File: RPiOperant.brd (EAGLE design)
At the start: 136 x 94 mm, 69 parts, among them IC1 74LS14N, IC2 74LS14N, J2 POWER_JACK

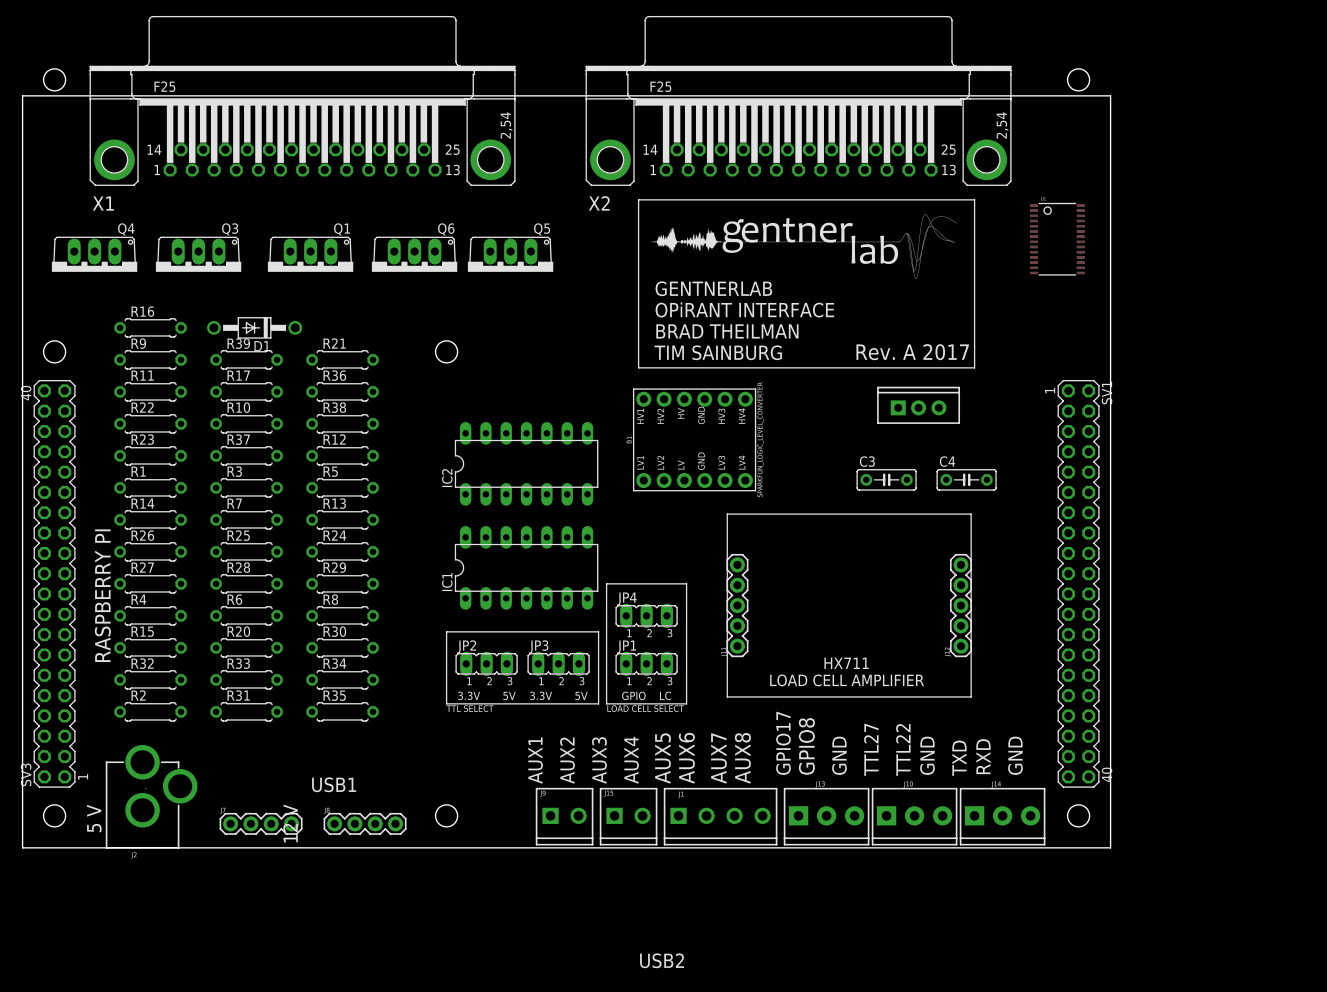
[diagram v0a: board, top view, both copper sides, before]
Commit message: new board layout
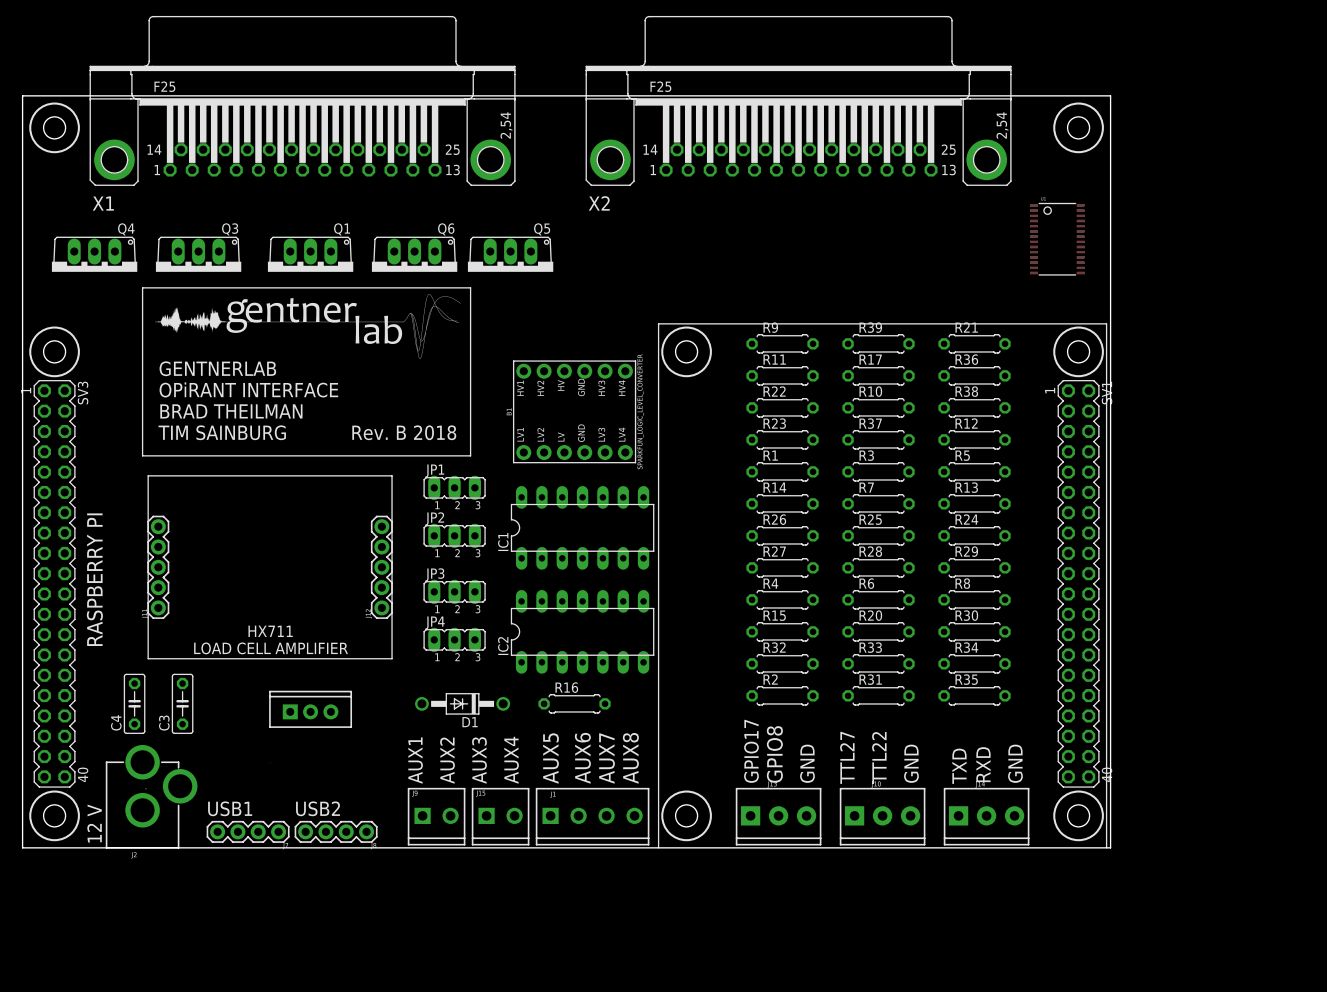
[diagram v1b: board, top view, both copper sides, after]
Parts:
- moved C4 107.7 mm to (14.0, 18.0), turned to 90 degrees
- moved C3 92.3 mm to (20.0, 18.0), turned to 90 degrees
- moved U2 85.0 mm to (36.0, 17.0)
- moved R1 79.0 mm to (95.0, 47.0)
- moved R10 79.0 mm to (107.0, 55.0)
- moved R11 79.0 mm to (95.0, 59.0)
- moved R12 79.0 mm to (119.0, 51.0)
- moved R13 79.0 mm to (119.0, 43.0)
- moved R14 79.0 mm to (95.0, 43.0)
- moved R15 79.0 mm to (95.0, 27.0)
- moved R17 79.0 mm to (107.0, 59.0)
- moved R2 79.0 mm to (95.0, 19.0)
- moved R20 79.0 mm to (107.0, 27.0)
- moved R21 79.0 mm to (119.0, 63.0)
- moved R22 79.0 mm to (95.0, 55.0)
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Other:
- board text added: "Rev. B 2018"
- board text removed: "3.3V 5V"
- board text removed: "5 V"
- board text removed: "GPIO LC"
- board text removed: "LOAD CELL SELECT"
- board text removed: "Rev. A 2017"
- board text removed: "TTL SELECT"

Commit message: revb revisions
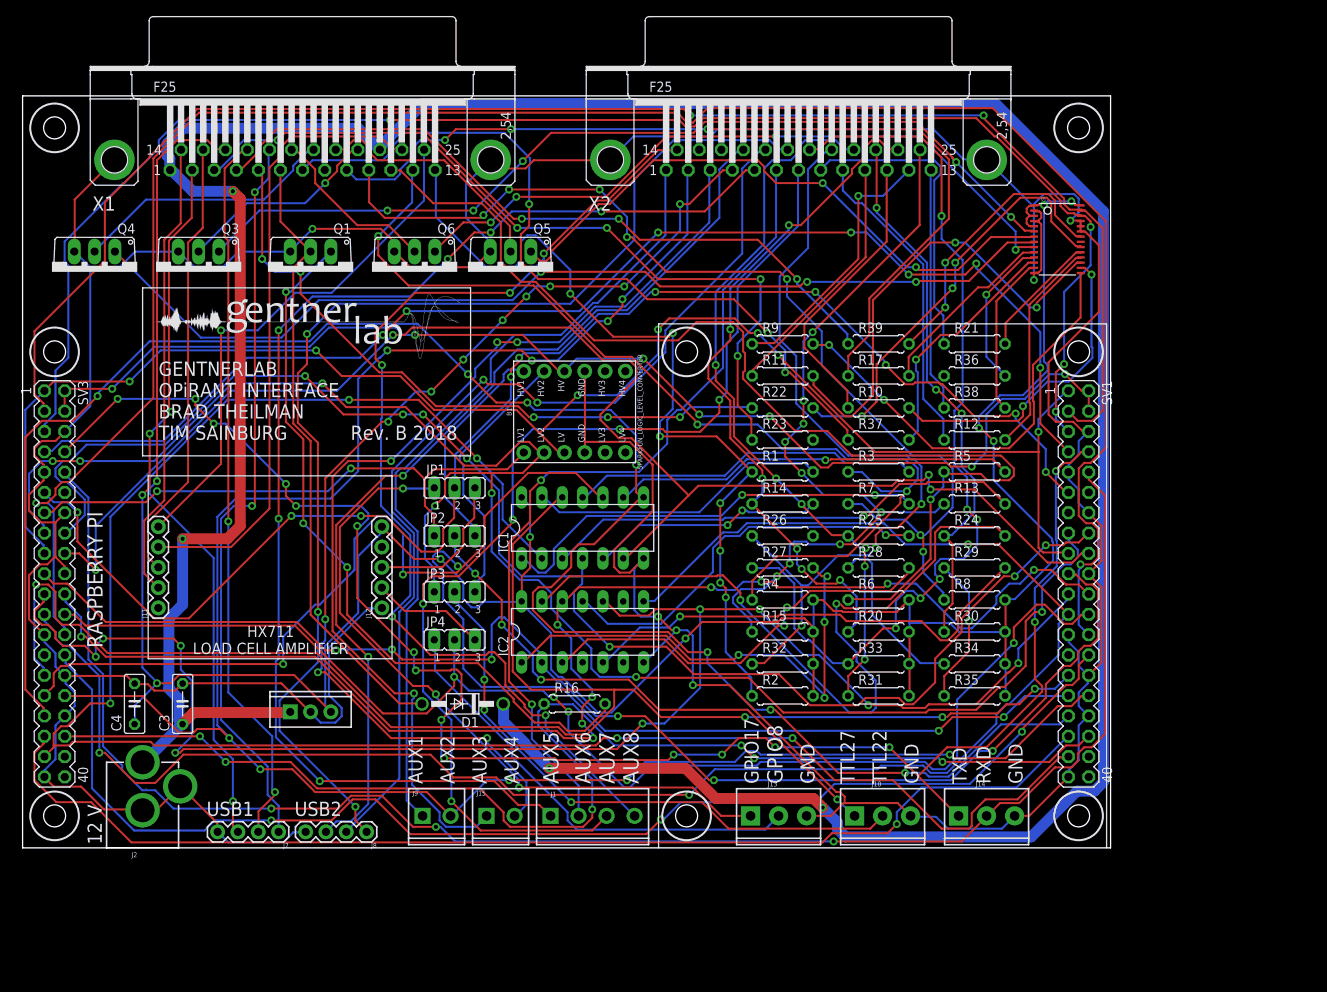
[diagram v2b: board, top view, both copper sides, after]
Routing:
- net GND: track 0.00 -> 590.5 mm, vias 0 -> 6
- net 12V: track 0.00 -> 393.1 mm, vias 0 -> 4
- net +3V3: track 0.00 -> 347.9 mm, vias 0 -> 11
- net AUX2: track 0.00 -> 259.7 mm, vias 0 -> 9
- net GPIO7: track 0.00 -> 255.2 mm, vias 0 -> 2
- net RIGHT_PECK_GPIO: track 0.00 -> 243.1 mm, vias 0 -> 5
- net CENTER_PECK_GPIO: track 0.00 -> 233.9 mm, vias 0 -> 7
- net GPIO22: track 0.00 -> 223.7 mm, vias 0 -> 7
- net IR_5_GPIO: track 0.00 -> 221.8 mm, vias 0 -> 3
- net TXD: track 0.00 -> 213.0 mm, vias 0 -> 16
- net RXD: track 0.00 -> 207.8 mm, vias 0 -> 3
- net LEFT_PECK_GPIO: track 0.00 -> 199.9 mm, vias 0 -> 5
- net RPI_3.3V: track 0.00 -> 197.2 mm, vias 0 -> 7
- net HOPPER_IR_GPIO: track 0.00 -> 196.0 mm, vias 0 -> 4
- net SCL: track 0.00 -> 195.5 mm, vias 0 -> 4
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
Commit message: new board!
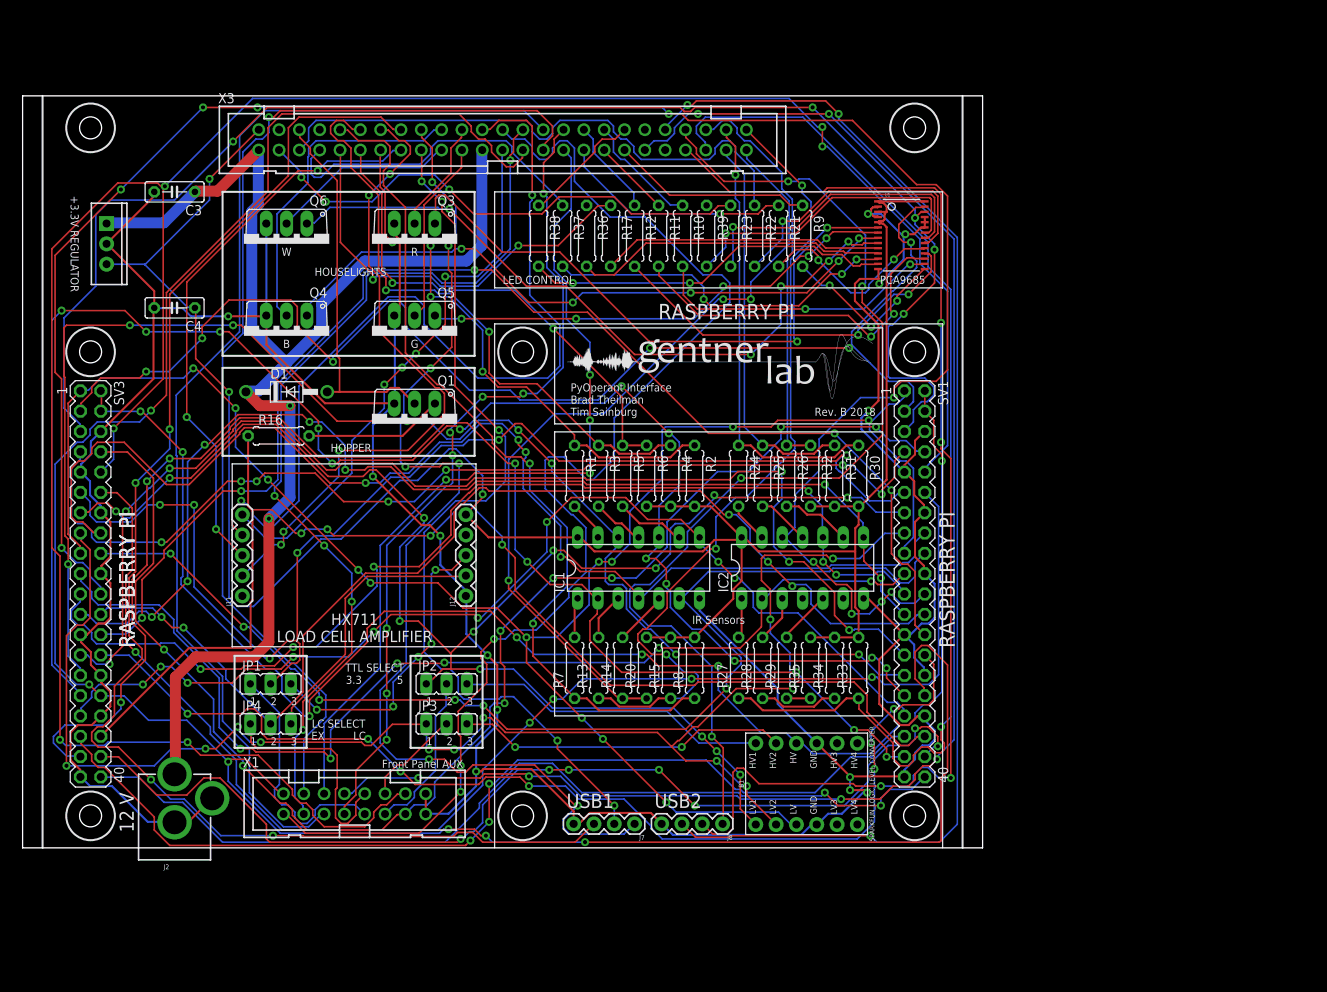
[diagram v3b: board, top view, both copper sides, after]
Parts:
- removed J1: (no value), SparkFun-Connectors:SCREWTERMINAL-3.5MM-4
- removed J10, J13, J14: (no value), SparkFun-Connectors:SCREWTERMINAL-3.5MM-3
- removed J15, J9: (no value), SparkFun-Connectors:SCREWTERMINAL-3.5MM-2
- removed X2: (no value), con-subd:F25HP
- added X3: 2550-, con-3m:PAK100/2500-50
- X1: value (none) -> 2516-; device con-subd:F25HP -> con-3m:PAK100/2500-16
- moved X1 80.8 mm to (41.5, 5.50)
- moved C3 64.0 mm to (19.0, 82.0), turned to 180 degrees
- moved U2 63.8 mm to (10.5, 75.5), turned to 270 degrees
- moved R38 58.6 mm to (64.5, 76.5), turned to 270 degrees
- moved B1 54.8 mm to (98.0, 8.00)
- moved R36 51.6 mm to (70.5, 76.5), turned to 270 degrees
- moved R13 51.3 mm to (72.0, 22.5), turned to 90 degrees
- moved R16 49.9 mm to (32.0, 51.5)
- moved C4 49.8 mm to (19.0, 67.5), turned to 180 degrees
- moved R12 49.6 mm to (76.5, 76.5), turned to 270 degrees
- moved R37 47.0 mm to (67.5, 76.5), turned to 270 degrees
- moved D1 44.8 mm to (33.0, 57.0), turned to 0 degrees
- moved J7 44.5 mm to (76.5, 3.00)
- moved J8 44.5 mm to (87.5, 3.00)
- moved R5 44.0 mm to (75.0, 46.5), turned to 270 degrees
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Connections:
- removed net N$32: J13.1, JP1.1
- removed net N$33: J13.2, JP4.1
- new net GPIO17EXT: JP1.1, X1.9
- new net GPIO8EXT: JP4.1, X1.10
- new net RGB_CUE_B\: X3.4
- net +3V3: now also X3.2; no longer X1.2
- net 12V: now also X3.1, X3.23; no longer X1.1, X1.23
- net AUX1: now also X1.1, X3.26; no longer J9.1, X2.1
- net AUX2: now also X1.2, X3.27; no longer J9.2, X2.2
- net AUX3: now also X1.3, X3.28; no longer J15.1, X2.3
- net AUX4: now also X1.4, X3.29; no longer J15.2, X2.4
- net AUX5: now also X1.5, X3.30; no longer J1.1, X2.5
- net AUX6: now also X1.6, X3.31; no longer J1.2, X2.6
- net AUX7: now also X1.7, X3.32; no longer J1.3, X2.7
- net AUX8: now also X1.8, X3.39; no longer J1.4, X2.14
- net CENTER_IR: now also X3.11; no longer X1.11
- net CENTER_LED: now also X3.8; no longer X1.8
- net GND: now also X1.15, X1.16; no longer J10.3, J13.3, J14.3, X1.G1, X1.G2, X2.G1, X2.G2
- net HOPPER: now also X3.6; no longer X1.6
- net HOPPER_IR: now also X3.13; no longer X1.13
- net HOUSELIGHT_B: now also X3.20; no longer X1.20
- net HOUSELIGHT_G: now also X3.21; no longer X1.21
- net HOUSELIGHT_R: now also X3.22; no longer X1.22
- net HOUSELIGHT_W: now also X3.19; no longer X1.19
- net IR_1: now also X3.50; no longer X2.25
- net IR_2: now also X3.49; no longer X2.24
- net IR_3: now also X3.48; no longer X2.23
- net IR_4: now also X3.47; no longer X2.22
- net IR_5: now also X3.46; no longer X2.21
- net IR_6: now also X3.45; no longer X2.20
- net LED_1: now also X3.38; no longer X2.13
- net LED_2: now also X3.37; no longer X2.12
- net LED_3: now also X3.36; no longer X2.11
- net LED_4: now also X3.35; no longer X2.10
- net LED_5: now also X3.34; no longer X2.9
- net LED_6: now also X3.33; no longer X2.8
- net LEFT_IR: now also X3.12; no longer X1.12
- net LEFT_LED: now also X3.9; no longer X1.9
- net LOADCELL2A+: now also X3.41; no longer X2.16
- net LOADCELL2A-: now also X3.40; no longer X2.15
- net LOADCELLA+: now also X3.15; no longer X1.15
- net LOADCELLA-: now also X3.14; no longer X1.14
- net LOADCELLE+: now also X3.25; no longer X1.25
- net LOADCELLE-: now also X3.24; no longer X1.24
- net RGB_CUE_B: no longer X1.4
- net RGB_CUE_G: now also X3.3; no longer X1.3
- net RGB_CUE_R: now also X3.5; no longer X1.5
- net RIGHT_IR: now also X3.10; no longer X1.10
- net RIGHT_LED: now also X3.7; no longer X1.7
- net RXD: now also X1.14; no longer J14.2
- net TTL22: now also X1.12; no longer J10.2
- net TTL27: now also X1.11; no longer J10.1
- net TXD: now also X1.13; no longer J14.1
- net USB1_D+: now also X3.16; no longer X1.16
- net USB1_D-: now also X3.17; no longer X1.17
- net USB1_VBUS: now also X3.18; no longer X1.18
- net USB2_D+: now also X3.42; no longer X2.17
- net USB2_D-: now also X3.43; no longer X2.18
- net USB2_VBUS: now also X3.44; no longer X2.19
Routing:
- net 12V: track 393.1 -> 165.0 mm, vias 4 -> 2
- net PCM_CLK: track 0.00 -> 168.9 mm, vias 0 -> 5
- net ID_SD: track 0.00 -> 149.3 mm, vias 0 -> 6
- net GPIO27: track 71.8 -> 201.3 mm, vias 2 -> 13
- net PCM_DIN: track 0.00 -> 128.8 mm, vias 0 -> 7
- net PCM_DOUT: track 0.00 -> 115.3 mm, vias 0 -> 2
- net GND: track 590.5 -> 475.2 mm, vias 6 -> 13
- net CENTER_PECK_GPIO: track 233.9 -> 132.7 mm, vias 7 -> 9
- net RXD: track 207.8 -> 308.8 mm, vias 3 -> 6
- net GPIO7: track 255.2 -> 161.4 mm, vias 2 -> 5
- net RGB_CUE_B: track 91.1 -> 0.00 mm, vias 3 -> 0
- net N$3: track 94.3 -> 5.09 mm, vias 2 -> 0
- net N$32: track 87.2 -> 0.00 mm, vias 3 -> 0
- net IR_3_GPIO: track 170.4 -> 251.6 mm, vias 9 -> 10
- net IR_5_GPIO: track 221.8 -> 140.6 mm, vias 3 -> 7
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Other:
- board size 136 x 94 mm -> 120 x 94 mm
- board text added: "+3.3V REGULATOR"
- board text added: "B"
- board text added: "Front Panel AUX"
- board text added: "G"
- board text added: "HOPPER"
- board text added: "HOUSELIGHTS"
- board text added: "IR Sensors"
- board text added: "LC SELECT EX LC"
- board text added: "LED CONTROL"
- board text added: "PCA9685"
- board text added: "PyOperant Interface Brad Theilman Tim Sainburg"
- board text added: "R"
- board text added: "TTL SELECT 3.3 5"
- board text added: "W"
- board text removed: "AUX1"
- board text removed: "AUX2"
- board text removed: "AUX3"
- board text removed: "AUX4"
- board text removed: "AUX5"
- board text removed: "AUX6"
- board text removed: "AUX7"
- board text removed: "AUX8"
- board text removed: "GENTNERLAB OPiRANT INTERFACE BRAD THEILMAN TIM SAINBURG"
- board text removed: "GND"
- board text removed: "GPIO17"
- board text removed: "GPIO8"
- board text removed: "RXD"
- board text removed: "TTL22"
- board text removed: "TTL27"
- board text removed: "TXD"

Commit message: new board
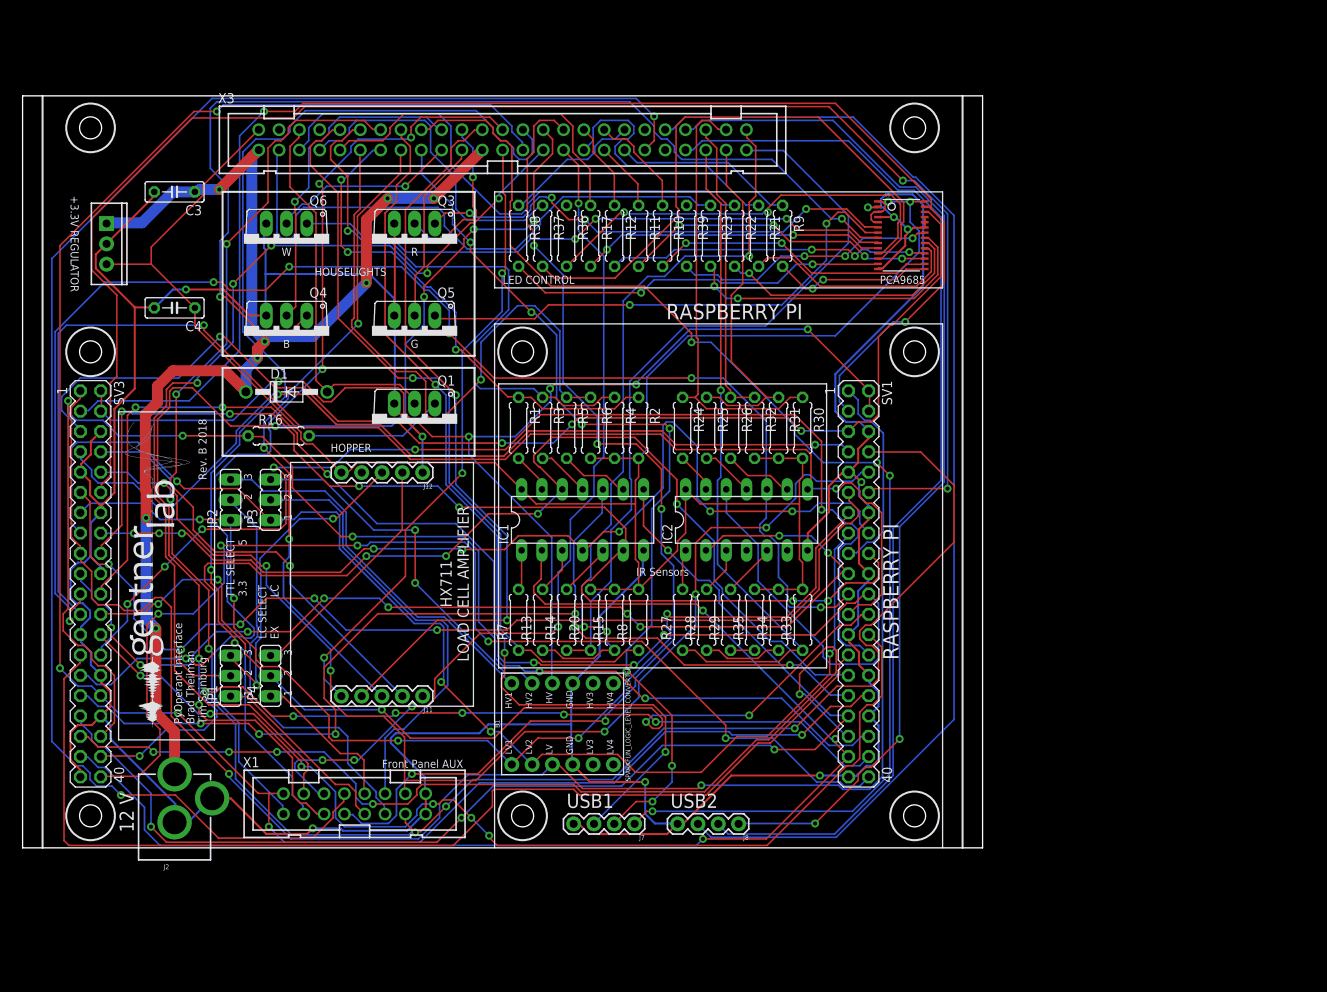
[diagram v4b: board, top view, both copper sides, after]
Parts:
- moved JP3 35.6 mm to (31.0, 43.5), turned to 90 degrees
- moved JP2 35.5 mm to (26.0, 43.5), turned to 90 degrees
- moved B1 31.4 mm to (67.5, 15.5)
- moved J11 25.8 mm to (50.0, 19.0), turned to 180 degrees
- moved J12 16.3 mm to (50.0, 46.9), turned to 180 degrees
- moved IC1 9.22 mm to (70.0, 41.0)
- moved IC2 9.22 mm to (90.5, 41.0)
- moved R1 9.22 mm to (62.0, 52.5)
- moved R13 9.22 mm to (65.0, 28.5)
- moved R14 9.22 mm to (68.0, 28.5)
- moved R15 9.22 mm to (74.0, 28.5)
- moved R2 9.22 mm to (77.0, 52.5)
- moved R20 9.22 mm to (71.0, 28.5)
- moved R24 9.22 mm to (82.5, 52.5)
- moved R25 9.22 mm to (85.5, 52.5)
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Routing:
- net RXD: track 308.8 -> 148.5 mm
- net LEFT_PECK_GPIO: track 203.8 -> 133.7 mm, vias 13 -> 6
- net IR_3_GPIO: track 251.6 -> 183.5 mm, vias 10 -> 6
- net GPIO27: track 201.3 -> 139.4 mm, vias 13 -> 5
- net USB1_D+: track 173.2 -> 116.9 mm, vias 4 -> 3
- net IR_6: track 138.8 -> 84.1 mm
- net HOUSELIGHT_B_GPIO: track 81.8 -> 130.1 mm, vias 5 -> 2
- net TTL22: track 12.5 -> 56.0 mm
- net IR_4_GPIO: track 134.5 -> 177.4 mm
- net AUX2: track 283.5 -> 243.6 mm, vias 6 -> 5
- net RPI_5V: track 193.7 -> 154.6 mm, vias 7 -> 5
- net GPIO22: track 191.3 -> 155.8 mm, vias 12 -> 4
- net AUX1: track 159.3 -> 124.5 mm
- net SCL: track 182.9 -> 148.9 mm, vias 5 -> 4
- net HOPPER_IR_GPIO: track 177.1 -> 144.3 mm, vias 8 -> 5
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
